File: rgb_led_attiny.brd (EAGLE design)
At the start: 57.6 x 55.8 mm, 14 parts, among them IC1 ATTINY45-20PU, IC2 MC7805BTG, Q1 IRF540NPBF, Q2 IRF540NPBF, Q3 IRF540NPBF

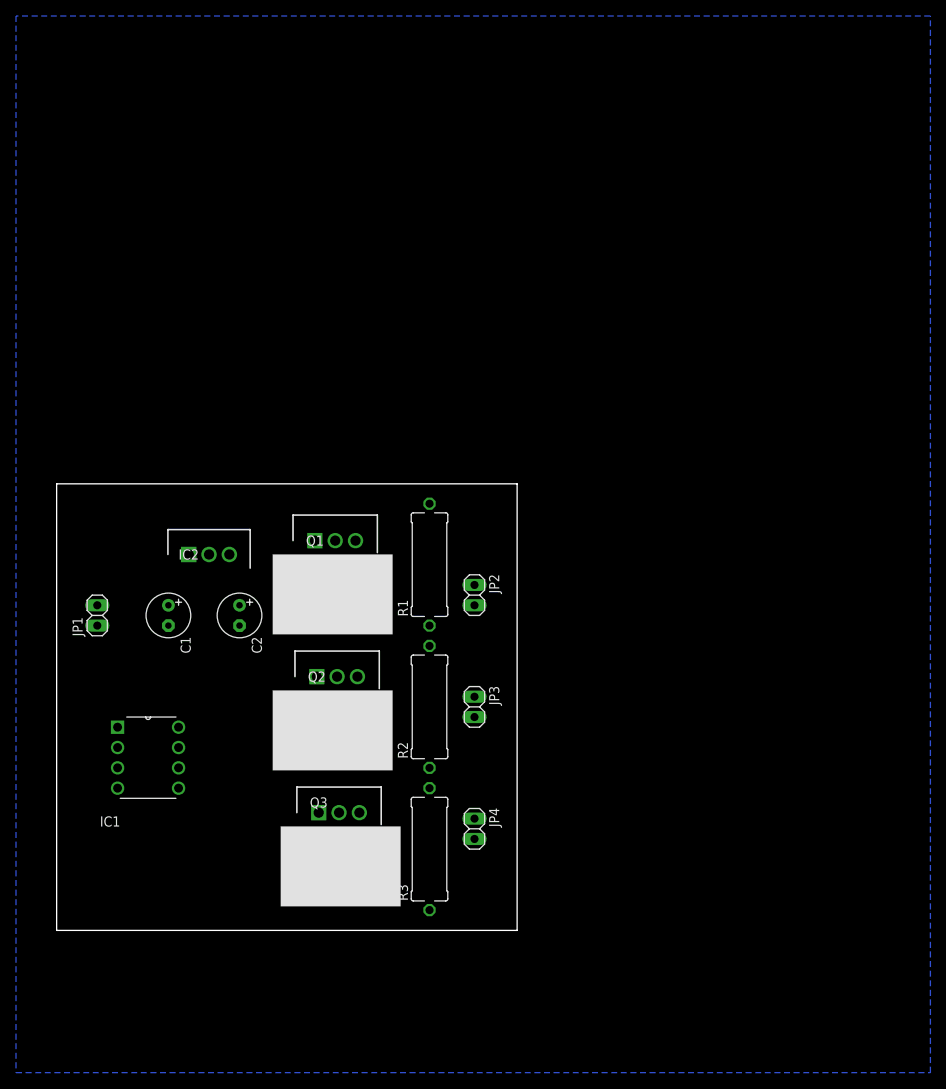
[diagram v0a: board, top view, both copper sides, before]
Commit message: Premier routage
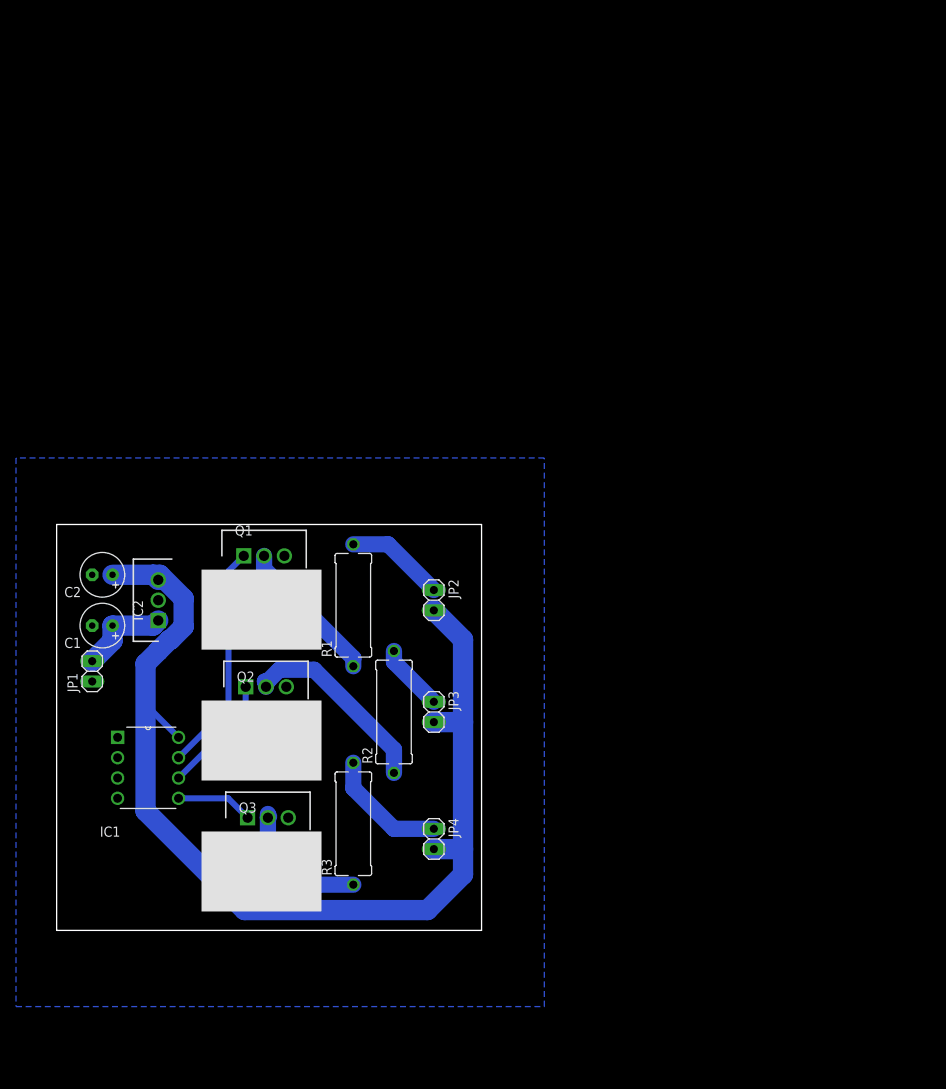
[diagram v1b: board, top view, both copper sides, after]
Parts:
- moved C2 17.9 mm to (5.71, 44.5), turned to 180 degrees
- moved R1 10.8 mm to (37.1, 40.6)
- moved R3 10.0 mm to (37.1, 13.3)
- moved IC2 9.09 mm to (12.7, 38.7), turned to 90 degrees
- moved Q1 9.09 mm to (23.4, 46.8)
- moved Q2 8.98 mm to (23.6, 30.4)
- moved Q3 8.91 mm to (23.9, 14.1)
- moved C1 8.35 mm to (5.71, 38.1), turned to 180 degrees
- moved JP1 7.01 mm to (4.45, 32.4)
- moved JP4 5.24 mm to (47.1, 11.4)
- moved JP2 5.12 mm to (47.1, 41.3)
- moved JP3 5.12 mm to (47.1, 27.3)
- moved R2 4.49 mm to (42.2, 27.3)
- moved IC1 1.27 mm to (15.2, 16.5)
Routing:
- net VCC: track 0.00 -> 139.0 mm
- net PWM_R: track 0.00 -> 28.6 mm
- net N$2: track 0.00 -> 24.5 mm
- net N$3: track 0.00 -> 18.4 mm
- net N$6: track 0.00 -> 16.6 mm
- net N$7: track 0.00 -> 15.3 mm
- net PWM_G: track 0.00 -> 14.9 mm
- net N$4: track 0.00 -> 12.4 mm
- net N$1: track 0.00 -> 11.5 mm
- net PWM_B: track 0.00 -> 9.63 mm
- net N$5: track 0.00 -> 8.41 mm
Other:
- board size 57.6 x 55.8 mm -> 53.1 x 50.7 mm
